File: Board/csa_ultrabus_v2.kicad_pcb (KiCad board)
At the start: 2 copper layers, 207.1 x 102.8 mm, 63 parts, among them IC1 7404D, IC2 74138D, IC3 74138D, IC4 74138D, IC5 74138D, IC6 7400D, IC7 74125D, IC8 74125D, IC9 74138D, J1 FLOP-4W827001, P1 CSABUSSOCK180, P2 CSABUSSOCK180, P3 CSABUSSOCK180, P4 CSABUSSOCK180, X1 PORT_EXPANSION_64_CONN

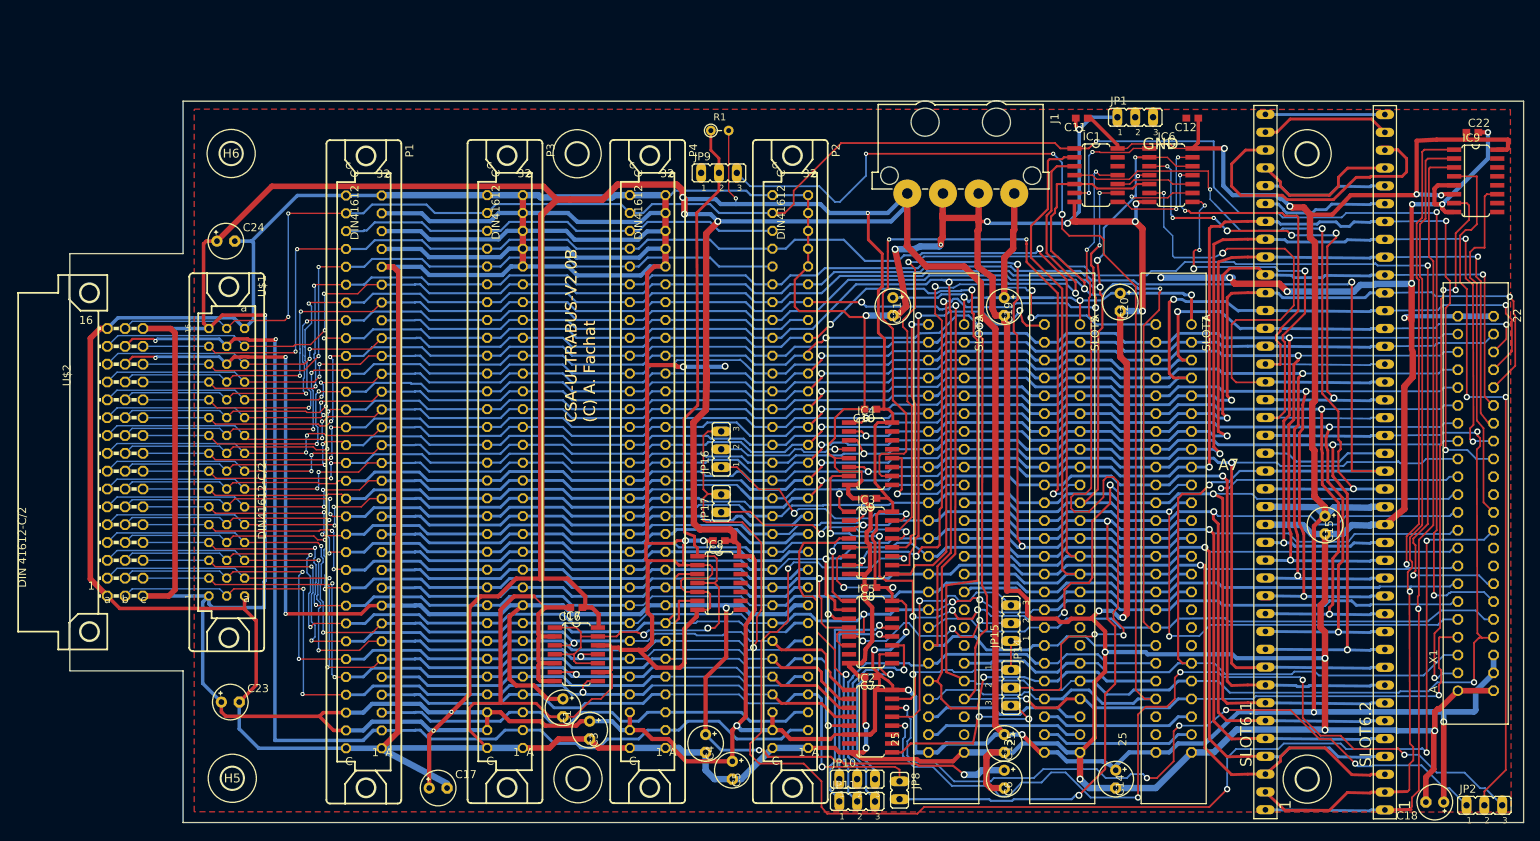
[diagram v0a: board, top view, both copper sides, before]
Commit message: layout ubus 2.1a
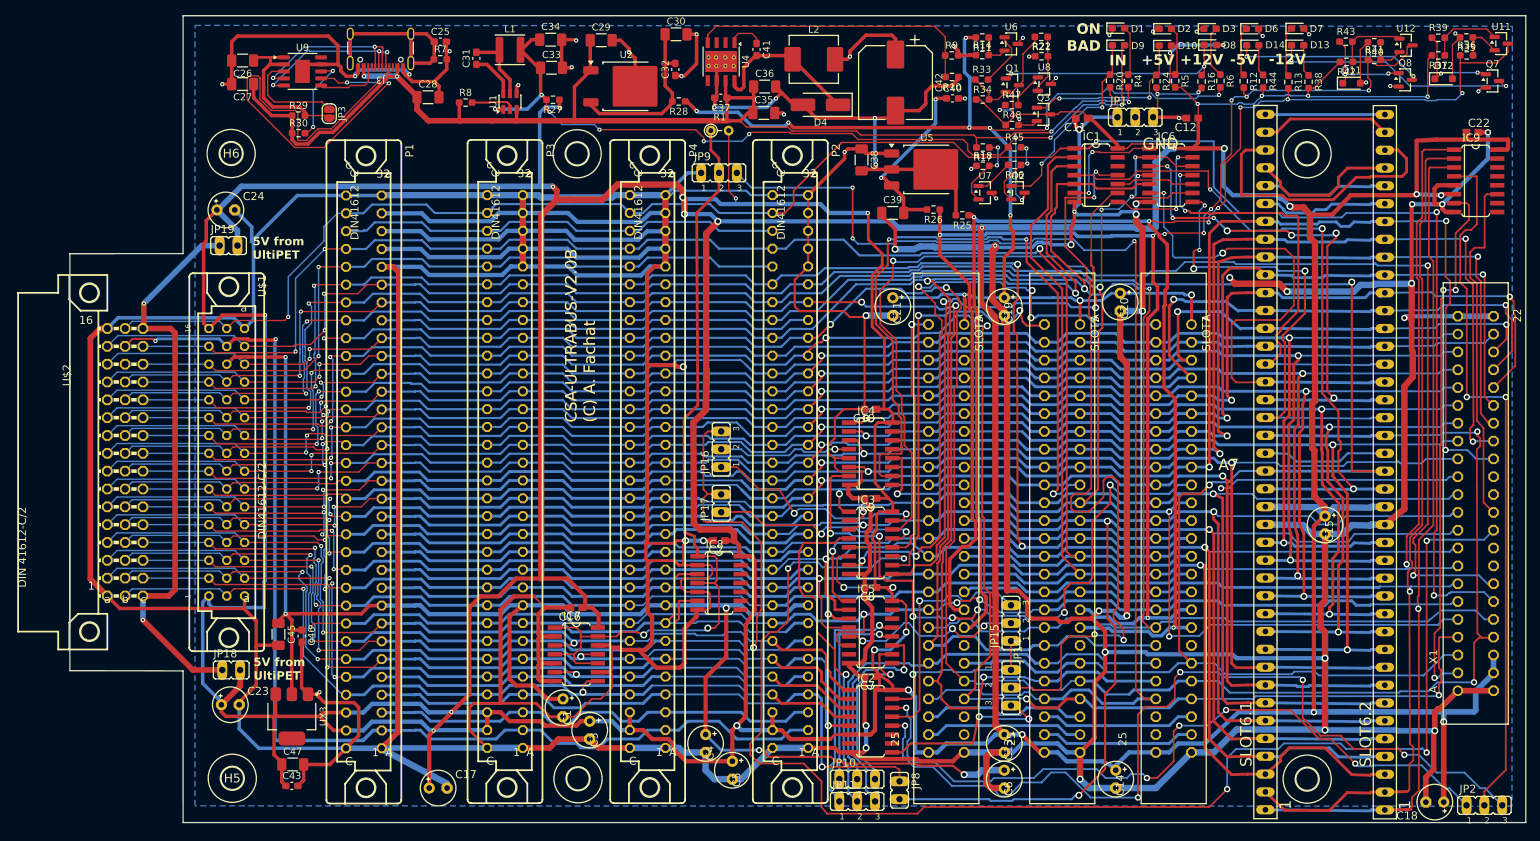
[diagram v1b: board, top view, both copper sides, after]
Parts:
- removed J1: FLOP-4W827001, csa_ultrabus_v2:827001
- added C25: 100n, Capacitor_SMD:C_0603_1608Metric_Pad1.08x0.95mm_HandSolder, F.Cu at (89.5, 43.7)
- added C26: 1u, Capacitor_SMD:C_1206_3216Metric_Pad1.33x1.80mm_HandSolder, F.Cu at (61.3, 46.4)
- added C27: 10u, Capacitor_SMD:C_1206_3216Metric_Pad1.33x1.80mm_HandSolder, F.Cu at (61.3, 49.8)
- added C28: 10u, Capacitor_SMD:C_1206_3216Metric_Pad1.33x1.80mm_HandSolder, F.Cu at (87.7, 51.6)
- added C29: 10u, Capacitor_SMD:C_1206_3216Metric_Pad1.33x1.80mm_HandSolder, F.Cu at (112.4, 43.5)
- added C30: 22u, Capacitor_SMD:C_1206_3216Metric_Pad1.33x1.80mm_HandSolder, F.Cu at (123.1, 42.7)
- added C31: 100n, Capacitor_SMD:C_0603_1608Metric_Pad1.08x0.95mm_HandSolder, F.Cu at (94.6, 46.1)
- added C32: 100n, Capacitor_SMD:C_0603_1608Metric_Pad1.08x0.95mm_HandSolder, F.Cu at (123.0, 47.7)
- added C33: 22u, Capacitor_SMD:C_1206_3216Metric_Pad1.33x1.80mm_HandSolder, F.Cu at (105.3, 47.4)
- added C34: 22u, Capacitor_SMD:C_1206_3216Metric_Pad1.33x1.80mm_HandSolder, F.Cu at (105.2, 43.4)
- added C35: 10u, Capacitor_SMD:C_1206_3216Metric_Pad1.33x1.80mm_HandSolder, F.Cu at (135.6, 53.9)
- added C36: 10u, Capacitor_SMD:C_1206_3216Metric_Pad1.33x1.80mm_HandSolder, F.Cu at (135.7, 50.1)
- added C37: 100n, Capacitor_SMD:C_0603_1608Metric_Pad1.08x0.95mm_HandSolder, F.Cu at (129.4, 51.7)
- added C38: 10u, Capacitor_SMD:C_1206_3216Metric_Pad1.33x1.80mm_HandSolder, F.Cu at (149.5, 60.6)
- added C39: 22u, Capacitor_SMD:C_1206_3216Metric_Pad1.33x1.80mm_HandSolder, F.Cu at (153.9, 68.1)
- added C40: 100n, Capacitor_SMD:C_0603_1608Metric_Pad1.08x0.95mm_HandSolder, F.Cu at (162.4, 51.8)
- added C41: 0.01uF low ESR, Capacitor_SMD:C_0603_1608Metric_Pad1.08x0.95mm_HandSolder, F.Cu at (134.5, 44.8)
- added C42: 220u, Capacitor_SMD:CP_Elec_10x10, F.Cu at (154.3, 49.5)
- added C43: 100n, Capacitor_SMD:C_0603_1608Metric_Pad1.08x0.95mm_HandSolder, F.Cu at (68.3, 149.7)
- added C45: 22u, Capacitor_SMD:C_1206_3216Metric_Pad1.33x1.80mm_HandSolder, F.Cu at (66.4, 128.1)
- added C46: 100n, Capacitor_SMD:C_0603_1608Metric_Pad1.08x0.95mm_HandSolder, F.Cu at (69.7, 128.4)
- added C47: 22u, Capacitor_SMD:C_1206_3216Metric_Pad1.33x1.80mm_HandSolder, F.Cu at (68.5, 146.7)
- added D1: LED, Diode_SMD:D_0603_1608Metric_Pad1.05x0.95mm_HandSolder, F.Cu at (186.1, 41.8)
- added D10: LED, Diode_SMD:D_0603_1608Metric_Pad1.05x0.95mm_HandSolder, F.Cu at (192.8, 44.3)
- added D11: 1N4148, Diode_SMD:D_SOD-323_HandSoldering, F.Cu at (219.3, 49.6)
- added D12: 1N4148, Diode_SMD:D_SOD-323_HandSoldering, F.Cu at (232.4, 49.0)
- added D13: LED, Diode_SMD:D_0603_1608Metric_Pad1.05x0.95mm_HandSolder, F.Cu at (211.6, 44.2)
- added D14: LED, Diode_SMD:D_0603_1608Metric_Pad1.05x0.95mm_HandSolder, F.Cu at (205.2, 44.2)
- added D2: LED, Diode_SMD:D_0603_1608Metric_Pad1.05x0.95mm_HandSolder, F.Cu at (192.8, 41.9)
- added D3: LED, Diode_SMD:D_0603_1608Metric_Pad1.05x0.95mm_HandSolder, F.Cu at (199.1, 41.9)
- added D4: B340A, Diode_SMD:D_SMA_Handsoldering, F.Cu at (143.6, 52.7)
- added D6: LED, Diode_SMD:D_0603_1608Metric_Pad1.05x0.95mm_HandSolder, F.Cu at (205.2, 41.9)
- added D7: LED, Diode_SMD:D_0603_1608Metric_Pad1.05x0.95mm_HandSolder, F.Cu at (211.6, 41.8)
- added D8: LED, Diode_SMD:D_0603_1608Metric_Pad1.05x0.95mm_HandSolder, F.Cu at (199.2, 44.2)
- added D9: LED, Diode_SMD:D_0603_1608Metric_Pad1.05x0.95mm_HandSolder, F.Cu at (186.1, 44.2)
- added J3: USB_C_Receptacle_USB2.0_16P, Connector_USB:USB_C_Receptacle_GCT_USB4105-xx-A_16P_TopMnt_Horizontal, F.Cu at (81.0, 43.7)
- added JP18: JP1E, csa_ultrabus_v2:JP1, F.Cu at (59.7, 133.2)
- added JP19: JP1E, csa_ultrabus_v2:JP1, F.Cu at (59.3, 72.8)
- added JP3: Jumper_2_Open, Jumper:SolderJumper-2_P1.3mm_Open_RoundedPad1.0x1.5mm, F.Cu at (73.7, 54.0)
- added L1: 4.7uH, Inductor_SMD:L_APV_ANR4030, F.Cu at (99.4, 44.9)
- added L2: 15uH, Inductor_SMD:L_APV_APH0630, F.Cu at (142.7, 46.2)
- added Q1: BC857, Package_TO_SOT_SMD:SOT-23, F.Cu at (171.0, 49.9)
- added Q2: BC857, Package_TO_SOT_SMD:SOT-23, F.Cu at (171.8, 65.2)
- added Q3: BC857, Package_TO_SOT_SMD:SOT-23, F.Cu at (175.4, 54.1)
- added Q7: BC847, Package_TO_SOT_SMD:SOT-23, F.Cu at (239.4, 49.3)
- added Q8: BC847, Package_TO_SOT_SMD:SOT-23, F.Cu at (226.9, 49.2)
- added R10: 1.1k, Resistor_SMD:R_0603_1608Metric_Pad0.98x0.95mm_HandSolder, F.Cu at (162.4, 48.8)
- added R11: 36k, Resistor_SMD:R_0603_1608Metric_Pad0.98x0.95mm_HandSolder, F.Cu at (166.7, 43.1)
- added R12: 420, Resistor_SMD:R_0603_1608Metric_Pad0.98x0.95mm_HandSolder, F.Cu at (203.9, 49.4)
- added R13: 2k2, Resistor_SMD:R_0603_1608Metric_Pad0.98x0.95mm_HandSolder, F.Cu at (210.3, 49.5)
- added R14: 10k, Resistor_SMD:R_0603_1608Metric_Pad0.98x0.95mm_HandSolder, F.Cu at (166.7, 45.6)
- added R16: 680, Resistor_SMD:R_0603_1608Metric_Pad0.98x0.95mm_HandSolder, F.Cu at (197.9, 49.4)
- added R17: 47k, Resistor_SMD:R_0603_1608Metric_Pad0.98x0.95mm_HandSolder, F.Cu at (166.8, 58.8)
- added R18: 10k, Resistor_SMD:R_0603_1608Metric_Pad0.98x0.95mm_HandSolder, F.Cu at (166.8, 61.4)
- added R20: 680, Resistor_SMD:R_0603_1608Metric_Pad0.98x0.95mm_HandSolder, F.Cu at (184.9, 49.3)
- added R21: 8.2k, Resistor_SMD:R_0603_1608Metric_Pad0.98x0.95mm_HandSolder, F.Cu at (175.1, 43.0)
- added R22: 10k, Resistor_SMD:R_0603_1608Metric_Pad0.98x0.95mm_HandSolder, F.Cu at (175.1, 45.8)
- added R24: 680, Resistor_SMD:R_0603_1608Metric_Pad0.98x0.95mm_HandSolder, F.Cu at (191.5, 49.4)
- added R25: 0, Resistor_SMD:R_0603_1608Metric_Pad0.98x0.95mm_HandSolder, F.Cu at (163.8, 68.5)
- added R26: 0, Resistor_SMD:R_0603_1608Metric_Pad0.98x0.95mm_HandSolder, F.Cu at (159.7, 67.6)
- added R27: 0, Resistor_SMD:R_0603_1608Metric_Pad0.98x0.95mm_HandSolder, F.Cu at (105.5, 52.0)
- added R28: 0, Resistor_SMD:R_0603_1608Metric_Pad0.98x0.95mm_HandSolder, F.Cu at (123.4, 52.2)
- added R29: 1k, >=0.3W, Resistor_SMD:R_0603_1608Metric_Pad0.98x0.95mm_HandSolder, F.Cu at (69.3, 54.2)
- added R30: 10k, Resistor_SMD:R_0603_1608Metric_Pad0.98x0.95mm_HandSolder, F.Cu at (69.3, 56.8)
- added R33: 2k2, Resistor_SMD:R_0603_1608Metric_Pad0.98x0.95mm_HandSolder, F.Cu at (166.6, 49.1)
- added R34: 2k2, Resistor_SMD:R_0603_1608Metric_Pad0.98x0.95mm_HandSolder, F.Cu at (166.7, 52.0)
- added R35: 36k, Resistor_SMD:R_0603_1608Metric_Pad0.98x0.95mm_HandSolder, F.Cu at (235.6, 43.1)
- added R36: 10k, Resistor_SMD:R_0603_1608Metric_Pad0.98x0.95mm_HandSolder, F.Cu at (235.7, 45.7)
- added R37: 2.2k, Resistor_SMD:R_0603_1608Metric_Pad0.98x0.95mm_HandSolder, F.Cu at (231.6, 45.7)
- added R38: 560, Resistor_SMD:R_0603_1608Metric_Pad0.98x0.95mm_HandSolder, F.Cu at (213.2, 49.4)
- added R39: 10k, Resistor_SMD:R_0603_1608Metric_Pad0.98x0.95mm_HandSolder, F.Cu at (231.6, 43.2)
- added R4: 3k3, Resistor_SMD:R_0603_1608Metric_Pad0.98x0.95mm_HandSolder, F.Cu at (187.5, 49.3)
- added R40: 8.6k, Resistor_SMD:R_0603_1608Metric_Pad0.98x0.95mm_HandSolder, F.Cu at (222.5, 43.8)
- added R41: 10k, Resistor_SMD:R_0603_1608Metric_Pad0.98x0.95mm_HandSolder, F.Cu at (222.5, 46.3)
- added R42: 2.2k, Resistor_SMD:R_0603_1608Metric_Pad0.98x0.95mm_HandSolder, F.Cu at (218.6, 46.6)
- added R43: 10k, Resistor_SMD:R_0603_1608Metric_Pad0.98x0.95mm_HandSolder, F.Cu at (218.5, 43.7)
- added R44: 560, Resistor_SMD:R_0603_1608Metric_Pad0.98x0.95mm_HandSolder, F.Cu at (206.7, 49.4)
- added R45: 2k2, Resistor_SMD:R_0603_1608Metric_Pad0.98x0.95mm_HandSolder, F.Cu at (171.3, 58.8)
- added R46: 2k2, Resistor_SMD:R_0603_1608Metric_Pad0.98x0.95mm_HandSolder, F.Cu at (171.3, 61.3)
- added R47: 2k2, Resistor_SMD:R_0603_1608Metric_Pad0.98x0.95mm_HandSolder, F.Cu at (170.9, 52.8)
- added R48: 2k2, Resistor_SMD:R_0603_1608Metric_Pad0.98x0.95mm_HandSolder, F.Cu at (170.9, 55.6)
- added R5: 420, Resistor_SMD:R_0603_1608Metric_Pad0.98x0.95mm_HandSolder, F.Cu at (194.2, 49.3)
- added R6: 2k2, Resistor_SMD:R_0603_1608Metric_Pad0.98x0.95mm_HandSolder, F.Cu at (200.6, 49.3)
- added R7: 5.1k, Resistor_SMD:R_0603_1608Metric_Pad0.98x0.95mm_HandSolder, F.Cu at (89.5, 46.2)
- added R8: 100k, Resistor_SMD:R_0603_1608Metric_Pad0.98x0.95mm_HandSolder, F.Cu at (93.1, 52.4)
- added R9: 10k, Resistor_SMD:R_0603_1608Metric_Pad0.98x0.95mm_HandSolder, F.Cu at (162.3, 45.7)
- added U1: AP63205WU, Package_TO_SOT_SMD:TSOT-23-6, F.Cu at (99.4, 52.2)
- added U11: TL431, Package_TO_SOT_SMD:SOT-23, F.Cu at (240.6, 44.0)
- added U12: TL431, Package_TO_SOT_SMD:SOT-23, F.Cu at (227.0, 44.2)
- added U2: L7812, Package_TO_SOT_SMD:TO-252-2, F.Cu at (116.0, 50.1)
- added U4: TPS5430DDA, Package_SO:TI_SO-PowerPAD-8_ThermalVias, F.Cu at (129.5, 46.6)
- added U5: L7905, Package_TO_SOT_SMD:TO-252-3_TabPin2, F.Cu at (158.8, 61.9)
- added U6: TL431DBZ, Package_TO_SOT_SMD:SOT-23, F.Cu at (170.8, 44.0)
- added U7: TL431DBZ, Package_TO_SOT_SMD:SOT-23, F.Cu at (167.1, 65.2)
- added U8: TL431DBZ, Package_TO_SOT_SMD:SOT-23, F.Cu at (175.5, 49.8)
- added U9: CH224K, Package_SO:SSOP-10-1EP_3.9x4.9mm_P1mm_EP2.1x3.3mm, F.Cu at (69.8, 48.0)
- added UX3: LDI1117, Package_TO_SOT_SMD:SOT-223, F.Cu at (68.3, 139.8)
- moved C24 4.44 mm to (58.9, 67.7)
- moved C23 0.38 mm to (59.6, 138.2)
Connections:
- net /CS/A BUS/16MHZ renamed /CS/A BUS/16MHZ
- net /CS/A BUS/50HZ renamed /CS/A BUS/50HZ
- net /CS/A BUS/I2SCL renamed /CS/A BUS/I2SCL
- net /CS/A BUS/I2SDA renamed /CS/A BUS/I2SDA
- net /CS/A BUS/NOEXEC renamed /CS/A BUS/NOEXEC
- net /CS/A BUS/NOTMAPD renamed /CS/A BUS/NOTMAPD
- net /CS/A BUS/WPROT renamed /CS/A BUS/WPROT
- net /CS/A BUS//EXTIO renamed /CS/A BUS//EXTIO
- net /CS/A BUS//SO renamed /CS/A BUS//SO
- C1 pad +: VCC33 -> V33
- C10 pad 1: VCC -> 5V
- C11 pad 1: VCC -> 5V
- C12 pad 1: VCC -> 5V
- C13 pad +: VCC -> 5V
- C14 pad +: VCC -> 5V
- C15 pad +: VCC -> 5V
- C16 pad 1: VCC -> 5V
- C17 pad +: VCC -> 5V
- C18 pad +: VCC -> 5V
- C2 pad 1: VCC -> 5V
- C22 pad 1: VCC -> 5V
- C23 pad +: VCC -> 5V
- C24 pad +: VCC -> 5V
- C3 pad +: VCC -> 5V
- C4 pad +: VCC33 -> V33
- C5 pad +: VCC -> 5V
- C6 pad +: VCC33 -> V33
- C7 pad 1: VCC -> 5V
- C8 pad 1: VCC -> 5V
- C9 pad 1: VCC -> 5V
- IC1 pad 14: VCC -> 5V
- IC2 pad 16: VCC -> 5V
- IC2 pad 6: VCC -> 5V
- IC3 pad 16: VCC -> 5V
- IC3 pad 6: VCC -> 5V
- IC4 pad 16: VCC -> 5V
- IC5 pad 16: VCC -> 5V
- IC6 pad 14: VCC -> 5V
- IC7 pad 14: VCC -> 5V
- IC8 pad 14: VCC -> 5V
- IC9 pad 16: VCC -> 5V
- IC9 pad 6: VCC -> 5V
- P1 pad A9: VCC33 -> V33
- P1 pad C2: VCC -> 5V
- P1 pad C3: VCC -> 5V
- P2 pad A9: VCC33 -> V33
- P2 pad C2: VCC -> 5V
- P2 pad C3: VCC -> 5V
- P3 pad A9: VCC33 -> V33
- P3 pad C2: VCC -> 5V
- P3 pad C3: VCC -> 5V
- P4 pad A9: VCC33 -> V33
- P4 pad C2: VCC -> 5V
- P4 pad C3: VCC -> 5V
- R1 pad 2: VCC -> 5V
- SLOT3 pad 25: VCC -> 5V
- SLOT3 pad R: unconnected-(SLOT3--5V-PadR) -> -5V
- SLOT3 pad S: unconnected-(SLOT3--12V-PadS) -> -12V
- SLOT5 pad 25: VCC -> 5V
- SLOT5 pad R: unconnected-(SLOT5--5V-PadR) -> -5V
- SLOT5 pad S: unconnected-(SLOT5--12V-PadS) -> -12V
- SLOT6.1 pad 18: VCC -> 5V
- SLOT6.2 pad 18: VCC -> 5V
- SLOT7 pad 25: VCC -> 5V
- SLOT7 pad R: unconnected-(SLOT7--5V-PadR) -> -5V
- SLOT7 pad S: unconnected-(SLOT7--12V-PadS) -> -12V
- U$1 pad B14: VCC33 -> V33
- U$1 pad C1: VCC -> 5V
- U$1 pad C16: VCC -> 5V
- U$2 pad B14: VCC33 -> unconnected-(U$2-VCC33-PadB14)
- U$2 pad C1: VCC -> Net-(U$2-VCC)
- U$2 pad C16: VCC -> Net-(U$2-VCC)
- X1 pad 2: VCC -> 5V
- X1 pad 3: VCC -> 5V
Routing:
- net 5V: track 0.00 -> 1257.9 mm, vias 0 -> 31
- net VCC: track 1150.4 -> 0.00 mm, vias 21 -> 0
- net -12V: track 0.00 -> 239.3 mm, vias 0 -> 8
- net -5V: track 0.00 -> 229.0 mm, vias 0 -> 9
- net VCC33: track 224.0 -> 0.00 mm, vias 6 -> 0
- net V33: track 0.00 -> 223.5 mm, vias 0 -> 5
- net VBUS: track 0.00 -> 185.9 mm, vias 0 -> 4
- net GND: track 1477.2 -> 1658.2 mm, vias 30 -> 61
- net 5VP: track 0.00 -> 131.1 mm, vias 0 -> 10
- net 12V: track 71.6 -> 180.7 mm, vias 3 -> 11
- net Net-(U$2-VCC): track 0.00 -> 81.9 mm, vias 0 -> 2
- net /usbpd negative voltages/-12VP: track 0.00 -> 75.6 mm, vias 0 -> 4
- net Net-(J3-CC1): track 0.00 -> 73.0 mm, vias 0 -> 2
- net Net-(U4-VSENSE): track 0.00 -> 41.8 mm
- net Net-(D13-K): track 0.00 -> 35.6 mm, vias 0 -> 2
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- added copper zone on B.Cu, net GND
- removed copper zone on F.Cu, net GND
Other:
- board size 207.1 x 102.8 mm -> 207.4 x 114.9 mm
- board text added: "+12V"
- board text added: "+5V"
- board text added: "-12V"
- board text added: "-5V"
- board text added: "5V from UltiPET"
- board text added: "IN"
- board text added: "ON BAD"
